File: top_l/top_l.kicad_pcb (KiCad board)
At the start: 2 copper layers, 134.9 x 119.3 mm, 31 parts, among them SW1 SW_Push, SW10 SW_Push, SW11 SW_Push, SW12 SW_Push, SW13 SW_Push, SW14 SW_Push, SW15 SW_Push, SW16 SW_Push, SW17 SW_Push, SW18 SW_Push, SW19 SW_Push, SW2 SW_Push, SW20 SW_Push, SW21 SW_Push, SW22 SW_Push, SW23 SW_Push, SW24 SW_Push, SW25 SW_Push, SW26 SW_Push, SW27 SW_Push, SW3 SW_Push, SW4 SW_Push, SW5 SW_Push, SW6 SW_Push, SW7 SW_Push, SW8 SW_Push, SW9 SW_Push

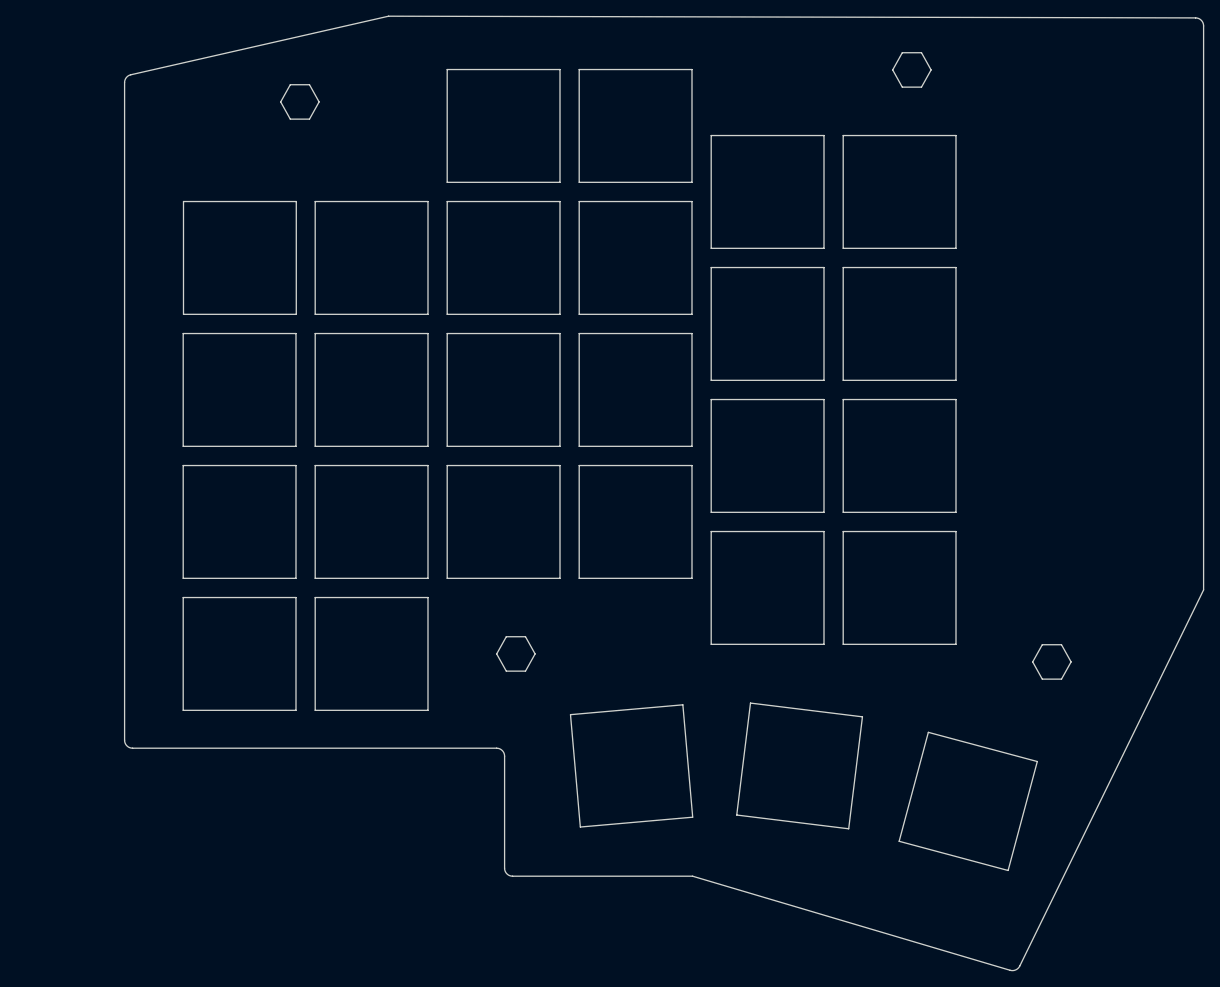
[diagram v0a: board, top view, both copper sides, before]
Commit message: refactor: top left plate
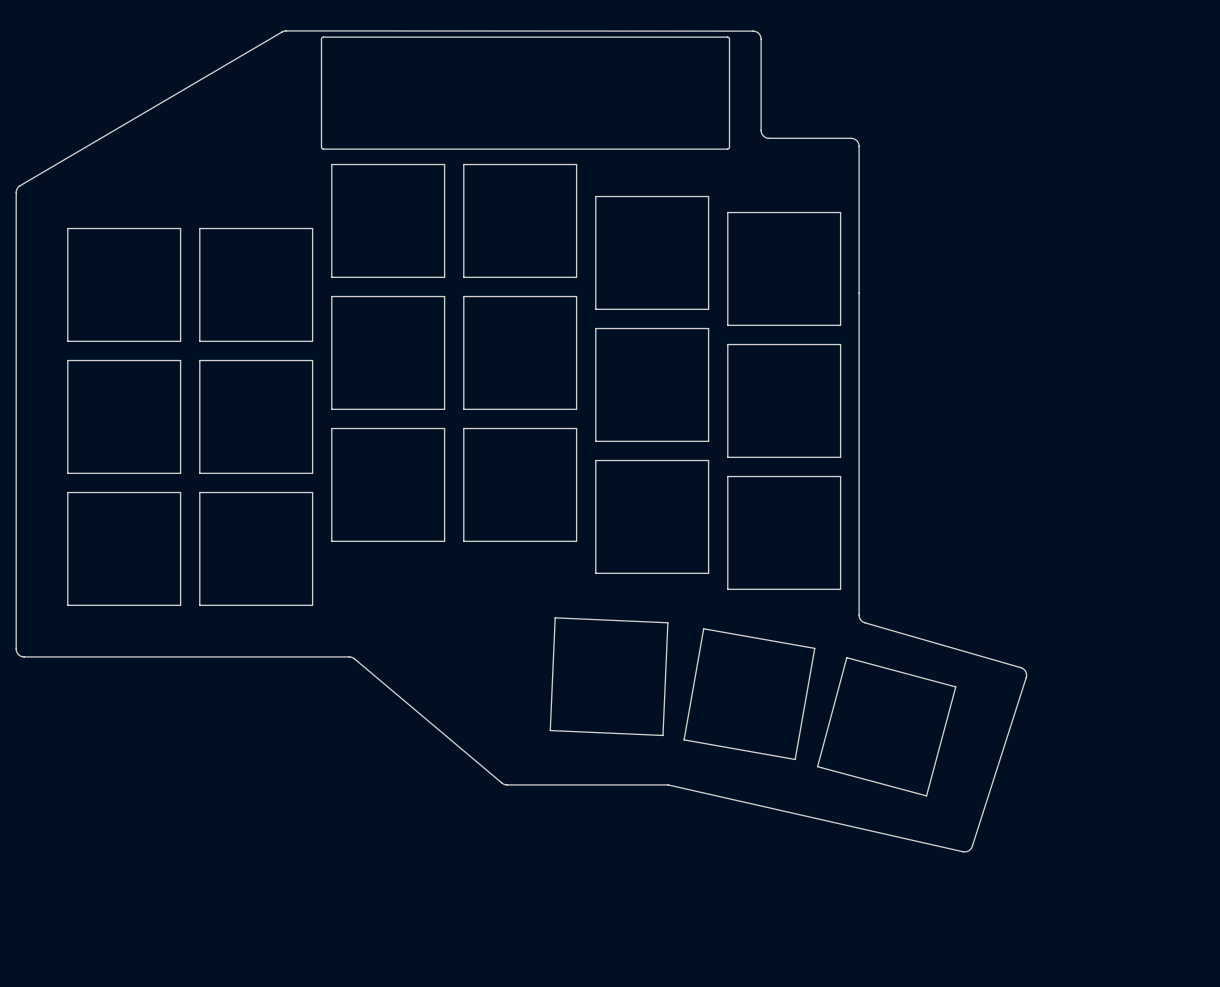
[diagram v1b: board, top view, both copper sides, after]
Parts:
- removed Ref** (x4): Val**, kbd_Hole:m2_Spacer_Hole_hex
- removed SW22, SW23, SW24, SW25, SW26, SW27: SW_Push, kbd_SW_Hole:SW_Hole_1u_16.5
- moved SW19 75.1 mm to (152.5, 87.9)
- moved SW3 71.0 mm to (70.0, 106.4), turned to 180 degrees
- moved SW5 69.8 mm to (86.5, 89.9)
- moved SW6 64.0 mm to (103.0, 65.4)
- moved SW21 54.3 mm to (165.3, 128.6), turned to -15 degrees
- moved SW20 53.7 mm to (152.5, 104.4)
- moved SW12 51.5 mm to (119.5, 98.4)
- moved SW4 51.4 mm to (86.5, 73.4)
- moved SW13 50.1 mm to (130.6, 122.3), turned to 177.5 degrees
- moved SW14 48.6 mm to (136.0, 69.4)
- moved SW9 47.7 mm to (86.5, 106.4)
- moved SW2 36.8 mm to (70.0, 89.9), turned to 180 degrees
- moved SW11 31.1 mm to (119.5, 81.9)
- moved SW17 29.9 mm to (148.2, 124.5), turned to -10 degrees
- moved SW18 27.5 mm to (152.5, 71.4)
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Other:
- board size 134.9 x 119.3 mm -> 126.3 x 102.6 mm
